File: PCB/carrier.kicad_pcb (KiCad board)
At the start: 6 copper layers, 69.6 x 46.1 mm, 125 parts, among them J1 SODIMM-260_Split, J2 Micro_SD_Card_Det2, Q2 BSS138, Q3 BSS138, Q4 BC817-40, Q5 BSS138, SW1 SW_DIP_x04, U1 SN74LVC8T245, U2 SN74LVC8T245, U3 SN74LVC8T245, U4 RT9742GGJ5

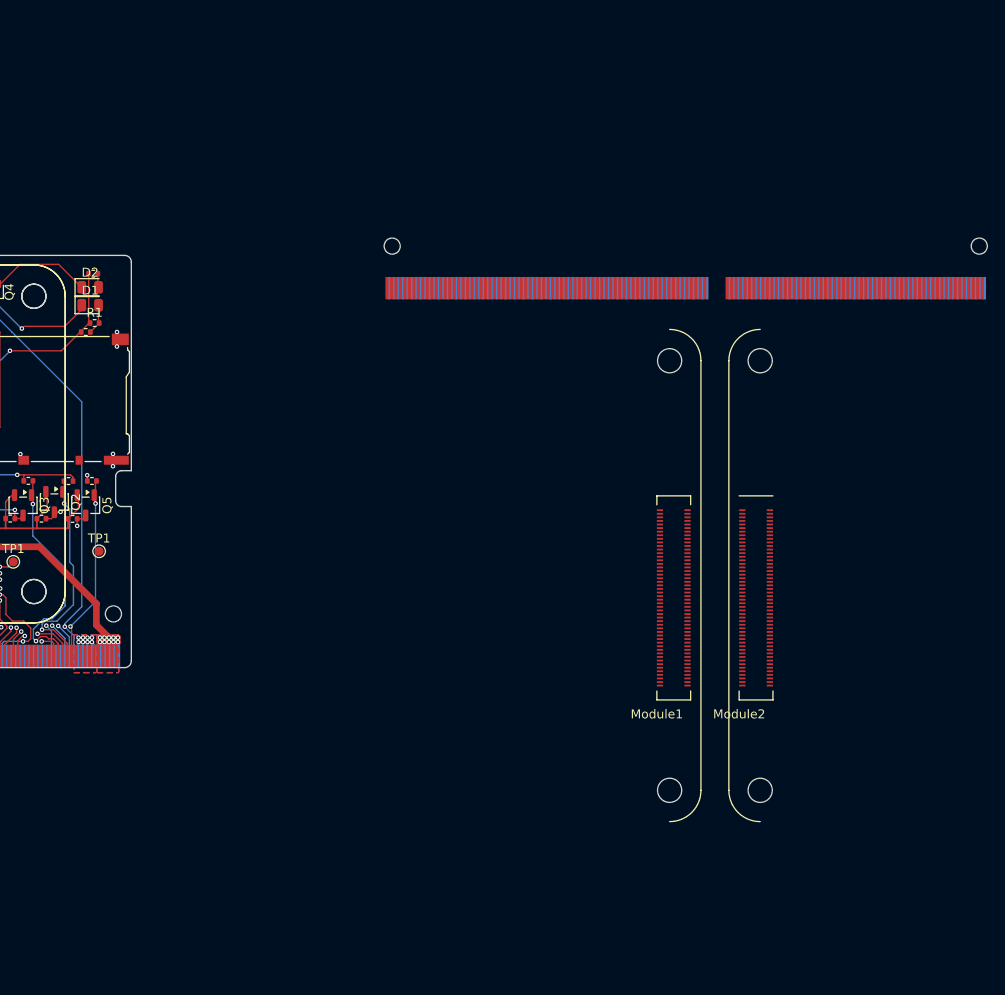
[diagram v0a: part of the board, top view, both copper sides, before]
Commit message: Place newly-added footprints on the board
Position SODIMM_DDR4_EDGE and the split CM4 mezzanine connector
footprints (Raspberry-Pi-4-Compute-Module-A/-B) at their board
locations now that the library links resolve correctly.

Co-Authored-By: Claude Sonnet 5 <noreply@anthropic.com>
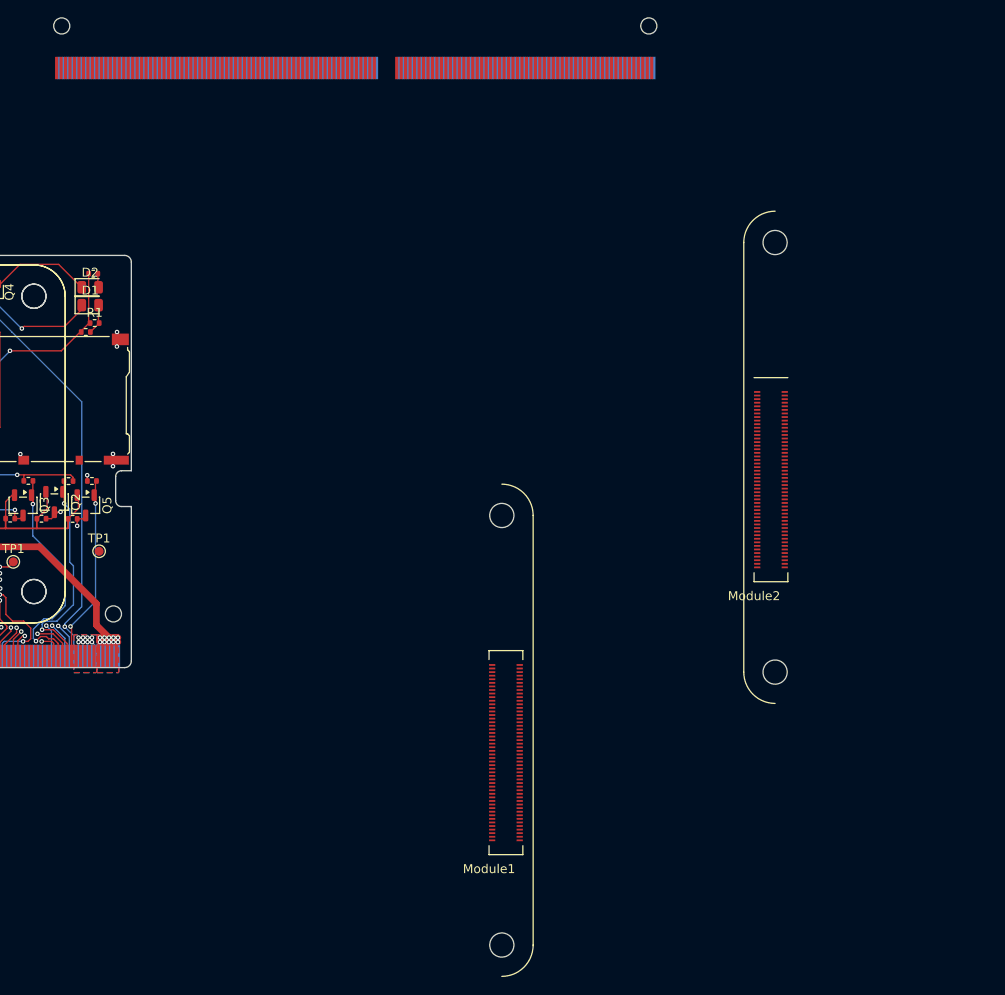
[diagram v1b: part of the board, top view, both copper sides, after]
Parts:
- moved J1 44.4 mm to (159.8, 34.3)
- moved Module1 25.5 mm to (178.0, 131.0)
- moved Module2 13.3 mm to (241.5, 100.5)
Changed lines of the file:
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@@
 	(footprint "CM4IO:Raspberry-Pi-4-Compute-Module-B"
 		(layer "F.Cu")
-		(at 196.75 113.71)
+		(at 178 131)
 		(descr "Raspberry Pi CM4 mezzanine connector B (J2, DF40C-100DS) - split from combined footprint, verify against datasheet before fab")
 		(tags "Raspberry Pi CM4 mezzanine connector B (J2, DF40C-100DS) - split from combined footprint, verify against datasheet before fab")
@@
 	(footprint "CM4IO:SODIMM_DDR4_EDGE"
 		(layer "F.Cu")
-		(at 196.75 58.9)
+		(at 159.825 34.3)
 		(descr "DDR4 SODIMM 260-pin card edge (gold finger) footprint, converted from legacy KiCad v4 source - VERIFY against JEDEC MO-310 / connector datasheet before fab")
 		(tags "SODIMM DDR4 260 edge connector card edge")
@@
 	(footprint "CM4IO:Raspberry-Pi-4-Compute-Module-A"
 		(layer "F.Cu")
-		(at 239.87 113.71)
+		(at 241.535 100.5)
 		(descr "Raspberry Pi CM4 mezzanine connector A (J1, DF40C-100DS) - split from combined footprint, verify against datasheet before fab")
 		(tags "Raspberry Pi CM4 mezzanine connector A (J1, DF40C-100DS) - split from combined footprint, verify against datasheet before fab")
